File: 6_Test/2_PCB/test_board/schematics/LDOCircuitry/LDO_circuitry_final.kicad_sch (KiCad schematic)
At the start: 6 parts

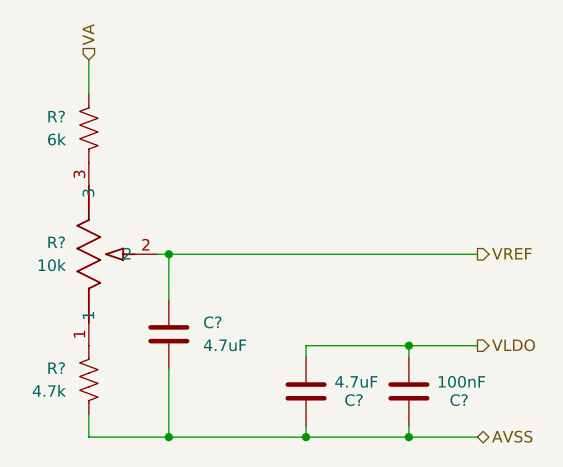
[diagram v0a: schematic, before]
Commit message: Corrections to schematic 11_20_24
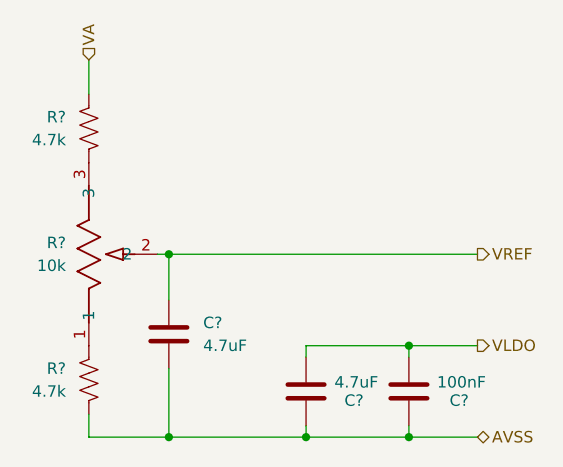
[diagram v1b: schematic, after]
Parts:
- R?: value 6k -> 4.7k
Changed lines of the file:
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@@
 				)
 			)
-			(project "LDO_circuitry_final"
-				(path "/9c0580c5-7bd5-4e54-bf4c-826aa4ac3630/104c40d7-ae25-447b-8675-a765b7f78bca"
-					(reference "C?")
+			(project "board_main"
+				(path "/9c0580c5-7bd5-4e54-bf4c-826aa4ac3630/104c40d7-ae25-447b-8675-a765b7f78bca"
+					(reference "C8")
 					(unit 1)
 				)
@@
 			)
 		)
-		(property "Value" "6k"
+		(property "Value" "4.7k"
 			(at 111.76 82.5499 0)
 			(effects
@@
 				)
 			)
-			(project "LDO_circuitry_final"
-				(path "/9c0580c5-7bd5-4e54-bf4c-826aa4ac3630/104c40d7-ae25-447b-8675-a765b7f78bca"
-					(reference "R?")
+			(project "board_main"
+				(path "/9c0580c5-7bd5-4e54-bf4c-826aa4ac3630/104c40d7-ae25-447b-8675-a765b7f78bca"
+					(reference "R7")
 					(unit 1)
 				)
@@
 				)
 			)
-			(project "LDO_circuitry_final"
-				(path "/9c0580c5-7bd5-4e54-bf4c-826aa4ac3630/104c40d7-ae25-447b-8675-a765b7f78bca"
-					(reference "C?")
+			(project "board_main"
+				(path "/9c0580c5-7bd5-4e54-bf4c-826aa4ac3630/104c40d7-ae25-447b-8675-a765b7f78bca"
+					(reference "C9")
 					(unit 1)
 				)
@@
 				)
 			)
-			(project "LDO_circuitry_final"
-				(path "/9c0580c5-7bd5-4e54-bf4c-826aa4ac3630/104c40d7-ae25-447b-8675-a765b7f78bca"
-					(reference "C?")
+			(project "board_main"
+				(path "/9c0580c5-7bd5-4e54-bf4c-826aa4ac3630/104c40d7-ae25-447b-8675-a765b7f78bca"
+					(reference "C7")
 					(unit 1)
 				)
@@
 				)
 			)
-			(project "LDO_circuitry_final"
-				(path "/9c0580c5-7bd5-4e54-bf4c-826aa4ac3630/104c40d7-ae25-447b-8675-a765b7f78bca"
-					(reference "R?")
+			(project "board_main"
+				(path "/9c0580c5-7bd5-4e54-bf4c-826aa4ac3630/104c40d7-ae25-447b-8675-a765b7f78bca"
+					(reference "R8")
 					(unit 1)
 				)
@@
 				)
 			)
-			(project "LDO_circuitry_final"
-				(path "/9c0580c5-7bd5-4e54-bf4c-826aa4ac3630/104c40d7-ae25-447b-8675-a765b7f78bca"
-					(reference "R?")
-					(unit 1)
-				)
+			(project "board_main"
+				(path "/9c0580c5-7bd5-4e54-bf4c-826aa4ac3630/104c40d7-ae25-447b-8675-a765b7f78bca"
+					(reference "R9")
+					(unit 1)
+				)
